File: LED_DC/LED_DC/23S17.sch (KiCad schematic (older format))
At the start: 20 parts, among them Q1 FDV304P, Q2 FDV304P, Q3 FDV304P, Q4 FDV304P, Q5 FDV304P, Q6 FDV304P, Q7 FDV304P, Q8 FDV304P, U1 74HC238, U2 ULN2803A

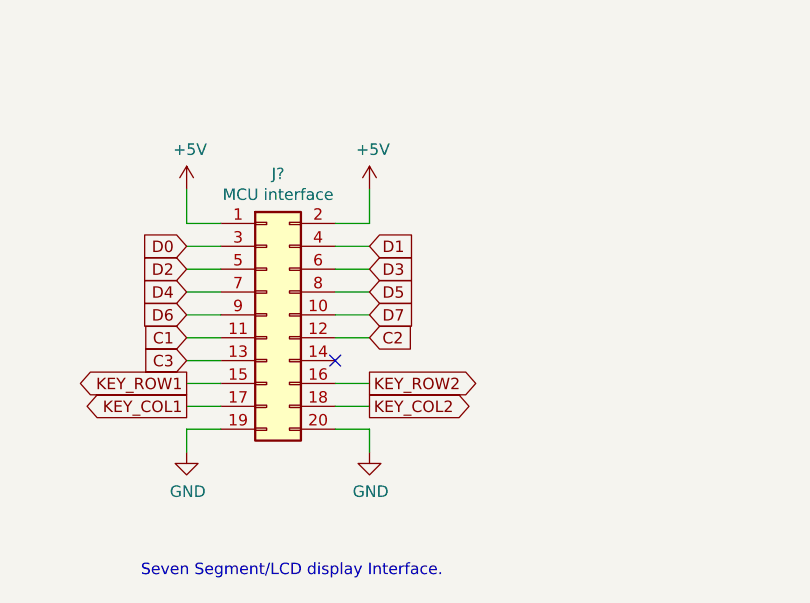
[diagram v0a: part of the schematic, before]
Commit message: Updated PCB.
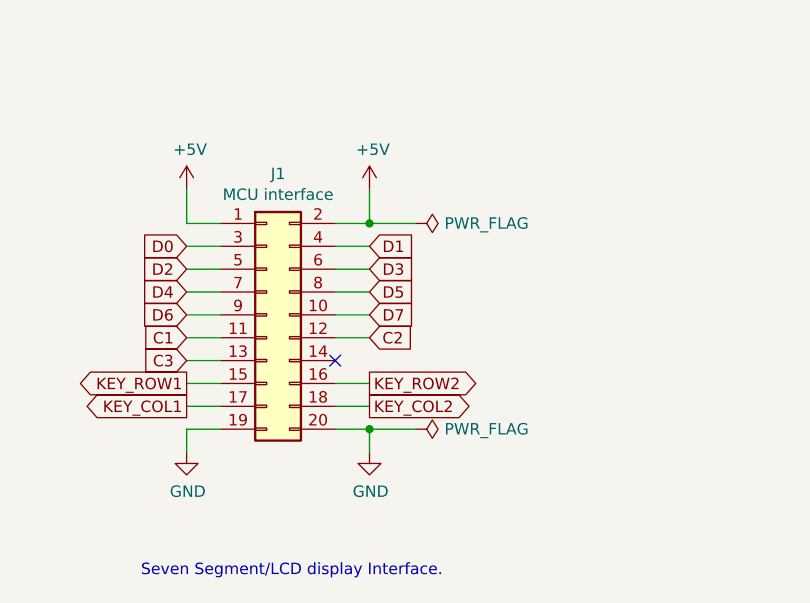
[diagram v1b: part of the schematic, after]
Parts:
- J1: renamed from J?; footprint (none) -> Connector_PinHeader_2.54mm:PinHeader_2x10_P2.54mm_Vertical
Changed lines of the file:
@@
 Seven Segment/LCD display Interface.
 $Comp
-L Connector_Generic:Conn_02x10_Odd_Even J?
+L Connector_Generic:Conn_02x10_Odd_Even J1
 U 1 1 6068829A
 P 2900 2950
-F 0 "J?" H 2950 3567 50  0000 C CNN
+F 0 "J1" H 2950 3567 50  0000 C CNN
 F 1 "MCU interface" H 2950 3476 50  0000 C CNN
-F 2 "" H 2900 2950 50  0001 C CNN
+F 2 "Connector_PinHeader_2.54mm:PinHeader_2x10_P2.54mm_Vertical" H 2900 2950 50  0001 C CNN
 F 3 "~" H 2900 2950 50  0001 C CNN
 	1    2900 2950
@@
 KEY_COL2
 $Comp
-L power:GND #PWR?
+L power:GND #PWR02
 U 1 1 60691F3F
 P 2550 3550
-F 0 "#PWR?" H 2550 3300 50  0001 C CNN
+F 0 "#PWR02" H 2550 3300 50  0001 C CNN
 F 1 "GND" H 2555 3377 50  0000 C CNN
 F 2 "" H 2550 3550 50  0001 C CNN
@@
 $EndComp
 $Comp
-L power:GND #PWR?
+L power:GND #PWR05
 U 1 1 60692355
 P 3350 3550
-F 0 "#PWR?" H 3350 3300 50  0001 C CNN
+F 0 "#PWR05" H 3350 3300 50  0001 C CNN
 F 1 "GND" H 3355 3377 50  0000 C CNN
 F 2 "" H 3350 3550 50  0001 C CNN
@@
 $EndComp
 $Comp
-L power:+5V #PWR?
+L power:+5V #PWR01
 U 1 1 60692883
 P 2550 2400
-F 0 "#PWR?" H 2550 2250 50  0001 C CNN
+F 0 "#PWR01" H 2550 2250 50  0001 C CNN
 F 1 "+5V" H 2565 2573 50  0000 C CNN
 F 2 "" H 2550 2400 50  0001 C CNN
@@
 $EndComp
 $Comp
-L power:+5V #PWR?
+L power:+5V #PWR03
 U 1 1 60692BF9
 P 3350 2400
-F 0 "#PWR?" H 3350 2250 50  0001 C CNN
+F 0 "#PWR03" H 3350 2250 50  0001 C CNN
 F 1 "+5V" H 3365 2573 50  0000 C CNN
 F 2 "" H 3350 2400 50  0001 C CNN
@@
 Wire Wire Line
 	3350 2650 3200 2650
+$Comp
+L power:PWR_FLAG #FLG0101
+U 1 1 606A139D
+P 3550 2550
+F 0 "#FLG0101" H 3550 2625 50  0001 C CNN
+F 1 "PWR_FLAG" V 3550 2678 50  0000 L CNN
+F 2 "" H 3550 2550 50  0001 C CNN
+F 3 "~" H 3550 2550 50  0001 C CNN
+	1    3550 2550
+	0    1    1    0
+$EndComp
+$Comp
+L power:PWR_FLAG #FLG0102
+U 1 1 606A16E2
+P 3550 3450
+F 0 "#FLG0102" H 3550 3525 50  0001 C CNN
+F 1 "PWR_FLAG" V 3550 3578 50  0000 L CNN
+F 2 "" H 3550 3450 50  0001 C CNN
+F 3 "~" H 3550 3450 50  0001 C CNN
+	1    3550 3450
+	0    1    1    0
+$EndComp
+Wire Wire Line
+	3550 3450 3350 3450
+Connection ~ 3350 3450
+Wire Wire Line
+	3350 2550 3550 2550
+Connection ~ 3350 2550
 $EndSCHEMATC
